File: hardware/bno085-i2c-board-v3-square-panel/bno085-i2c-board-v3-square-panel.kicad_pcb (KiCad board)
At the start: 2 copper layers, 60 x 76.5 mm, 200 parts, among them J5 Conn_01x04_Pin

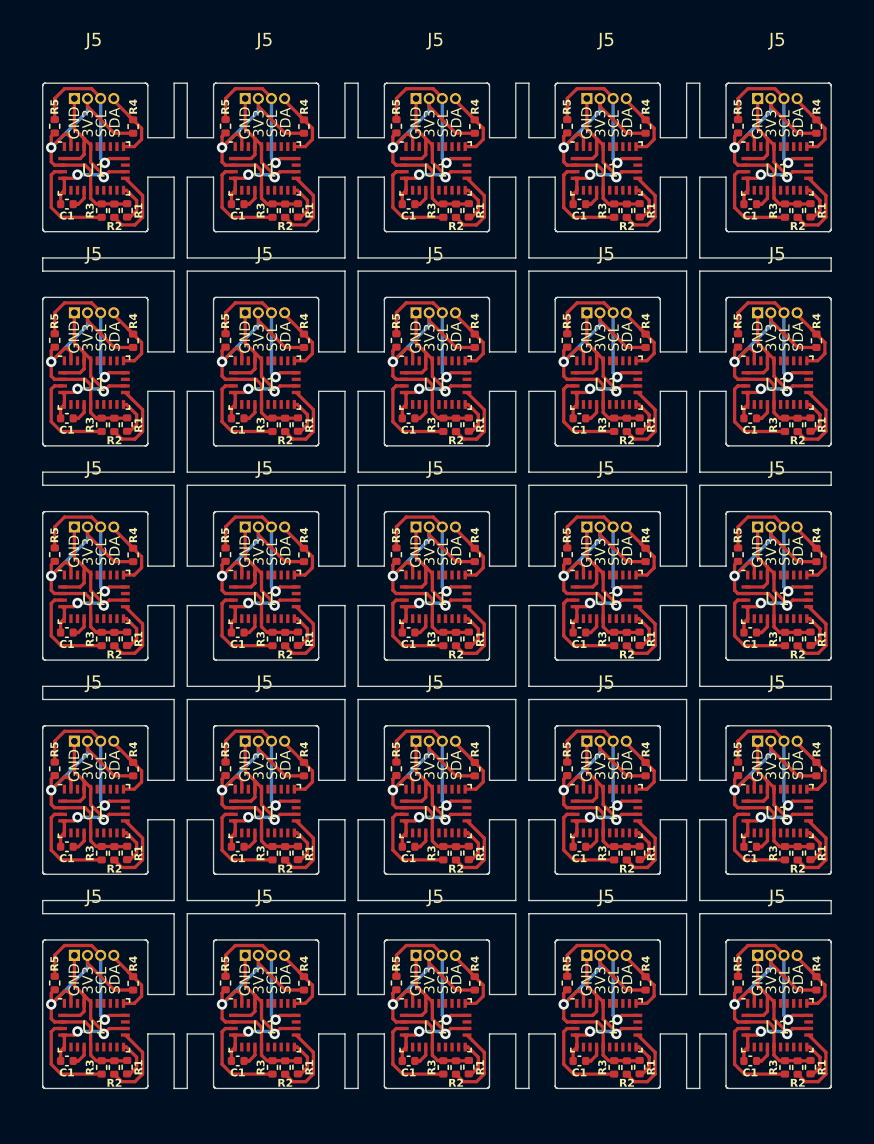
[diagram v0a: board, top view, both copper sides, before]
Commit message: square panel
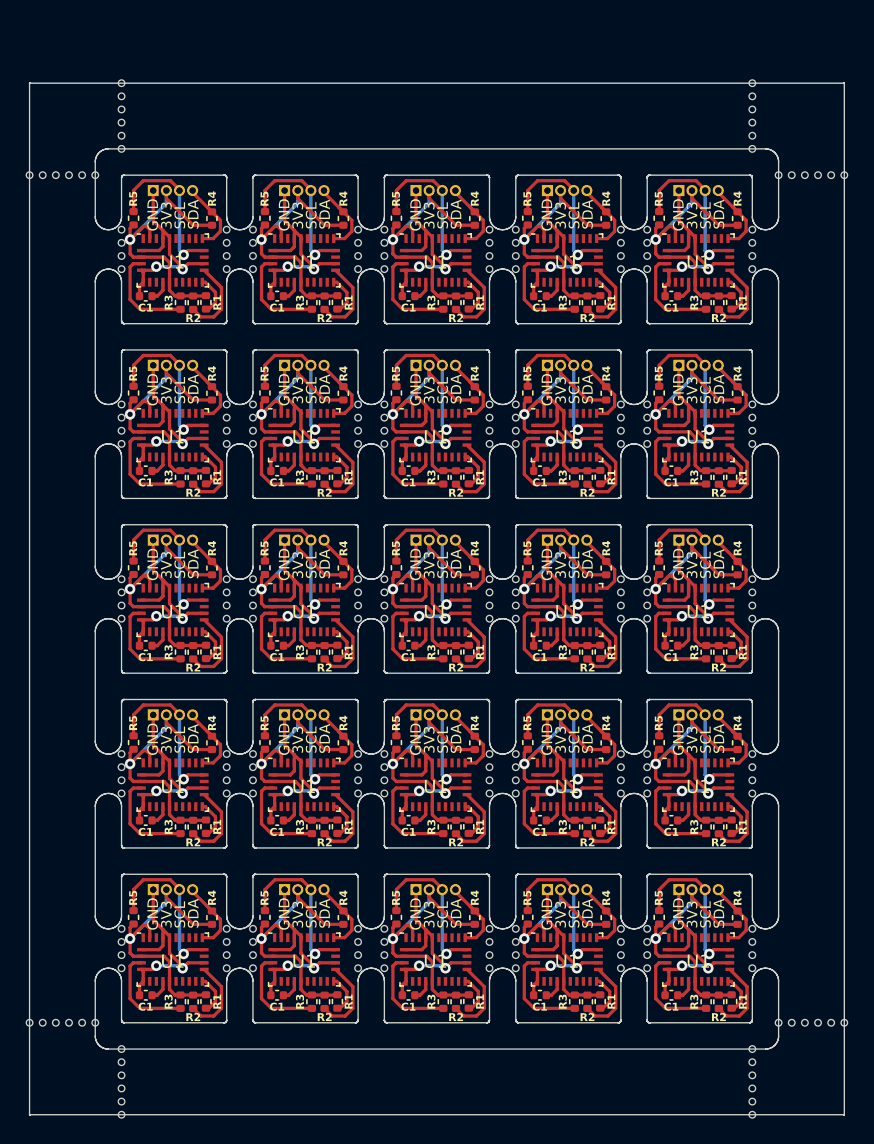
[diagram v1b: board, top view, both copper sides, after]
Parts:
- removed the C1 at (120.3, 29.2)
- removed the C1 at (172.3, 45.5)
- removed the C1 at (133.3, 94.4)
- removed the C1 at (133.3, 29.2)
- removed the C1 at (159.3, 78.1)
- removed the C1 at (159.3, 45.5)
- removed the C1 at (146.3, 94.4)
- removed the C1 at (159.3, 94.4)
- removed the C1 at (133.3, 78.1)
- removed the C1 at (133.3, 61.8)
- removed the C1 at (120.3, 61.8)
- removed the C1 at (120.3, 94.4)
- removed the C1 at (159.3, 29.2)
- removed the C1 at (172.3, 61.8)
- removed the C1 at (133.3, 45.5)
- removed the C1 at (172.3, 29.2)
- removed the C1 at (146.3, 45.5)
- removed the C1 at (120.3, 45.5)
- removed the C1 at (146.3, 61.8)
- removed the C1 at (172.3, 78.1)
- removed the C1 at (172.3, 94.4)
- removed the C1 at (146.3, 29.2)
- removed the C1 at (159.3, 61.8)
- removed the C1 at (120.3, 78.1)
- removed the C1 at (146.3, 78.1)
- removed the J5 at (172.9, 53.8)
- removed the J5 at (159.9, 37.5)
- removed the J5 at (159.9, 53.8)
- removed the J5 at (133.9, 53.8)
- removed the J5 at (120.9, 37.5)
- removed the J5 at (133.9, 37.5)
- removed the J5 at (133.9, 86.4)
- removed the J5 at (146.9, 86.4)
- removed the J5 at (172.9, 86.4)
- removed the J5 at (146.9, 53.8)
- removed the J5 at (172.9, 21.2)
- removed the J5 at (172.9, 70.1)
- removed the J5 at (146.9, 70.1)
- removed the J5 at (159.9, 70.1)
- removed the J5 at (120.9, 53.8)
- removed the J5 at (133.9, 21.2)
- removed the J5 at (120.9, 21.2)
- removed the J5 at (172.9, 37.5)
- removed the J5 at (120.9, 70.1)
- removed the J5 at (133.9, 70.1)
- removed the J5 at (146.9, 21.2)
- removed the J5 at (159.9, 86.4)
- removed the J5 at (120.9, 86.4)
- removed the J5 at (159.9, 21.2)
- removed the J5 at (146.9, 37.5)
- removed the R1 at (150.9, 78.6)
- removed the R1 at (163.9, 46.0)
- removed the R1 at (163.9, 62.3)
- removed the R1 at (124.9, 29.7)
- removed the R1 at (137.9, 78.6)
- removed the R1 at (124.9, 46.0)
- removed the R1 at (137.9, 46.0)
- removed the R1 at (176.9, 46.0)
- removed the R1 at (137.9, 62.3)
- removed the R1 at (124.9, 78.6)
- removed the R1 at (163.9, 78.6)
- removed the R1 at (150.9, 62.3)
- removed the R1 at (176.9, 29.7)
- removed the R1 at (163.9, 29.7)
- removed the R1 at (176.9, 78.6)
- removed the R1 at (150.9, 29.7)
- removed the R1 at (176.9, 94.9)
- removed the R1 at (176.9, 62.3)
- removed the R1 at (137.9, 29.7)
- removed the R1 at (150.9, 94.9)
- removed the R1 at (163.9, 94.9)
- removed the R1 at (124.9, 62.3)
- removed the R1 at (150.9, 46.0)
- removed the R1 at (124.9, 94.9)
- removed the R1 at (137.9, 94.9)
- removed the R2 at (163.0, 94.9)
- removed the R2 at (124.0, 46.0)
- removed the R2 at (124.0, 94.9)
- removed the R2 at (137.0, 46.0)
- removed the R2 at (137.0, 29.7)
- removed the R2 at (150.0, 94.9)
- removed the R2 at (176.0, 94.9)
- removed the R2 at (137.0, 62.3)
- removed the R2 at (124.0, 62.3)
- removed the R2 at (150.0, 29.7)
- removed the R2 at (176.0, 78.6)
- removed the R2 at (176.0, 46.0)
- removed the R2 at (137.0, 94.9)
- removed the R2 at (150.0, 78.6)
- removed the R2 at (124.0, 78.6)
- removed the R2 at (163.0, 46.0)
- removed the R2 at (150.0, 62.3)
- removed the R2 at (124.0, 29.7)
- removed the R2 at (163.0, 62.3)
- removed the R2 at (176.0, 62.3)
- removed the R2 at (163.0, 78.6)
- removed the R2 at (150.0, 46.0)
- removed the R2 at (137.0, 78.6)
- removed the R2 at (176.0, 29.7)
- removed the R2 at (163.0, 29.7)
- removed the R3 at (149.0, 94.9)
- removed the R3 at (149.0, 62.3)
- removed the R3 at (136.0, 29.7)
- removed the R3 at (162.0, 62.3)
- removed the R3 at (123.0, 62.3)
- removed the R3 at (149.0, 29.7)
- removed the R3 at (162.0, 29.7)
- removed the R3 at (123.0, 94.9)
- removed the R3 at (136.0, 94.9)
- removed the R3 at (175.0, 78.6)
- removed the R3 at (123.0, 46.0)
- removed the R3 at (123.0, 78.6)
- removed the R3 at (123.0, 29.7)
- removed the R3 at (175.0, 62.3)
- removed the R3 at (162.0, 78.6)
- removed the R3 at (136.0, 46.0)
- removed the R3 at (162.0, 46.0)
- removed the R3 at (175.0, 46.0)
- removed the R3 at (162.0, 94.9)
- removed the R3 at (149.0, 46.0)
- removed the R3 at (175.0, 94.9)
- removed the R3 at (136.0, 62.3)
- removed the R3 at (175.0, 29.7)
- removed the R3 at (149.0, 78.6)
- removed the R3 at (136.0, 78.6)
- removed the R4 at (164.4, 55.9)
- removed the R4 at (125.4, 55.9)
- removed the R4 at (164.4, 39.6)
- removed the R4 at (125.4, 88.5)
- removed the R4 at (125.4, 72.2)
- removed the R4 at (138.4, 39.6)
- removed the R4 at (177.4, 39.6)
- removed the R4 at (177.4, 23.3)
- removed the R4 at (151.4, 88.5)
- removed the R4 at (125.4, 23.3)
- removed the R4 at (151.4, 39.6)
- removed the R4 at (138.4, 23.3)
- removed the R4 at (151.4, 72.2)
- removed the R4 at (151.4, 55.9)
- removed the R4 at (177.4, 88.5)
- removed the R4 at (164.4, 72.2)
- removed the R4 at (177.4, 55.9)
- removed the R4 at (125.4, 39.6)
- removed the R4 at (151.4, 23.3)
- removed the R4 at (164.4, 23.3)
- removed the R4 at (138.4, 72.2)
- removed the R4 at (138.4, 88.5)
- removed the R4 at (177.4, 72.2)
- removed the R4 at (164.4, 88.5)
- removed the R4 at (138.4, 55.9)
- removed the R5 at (171.4, 55.9)
- removed the R5 at (132.4, 39.6)
- removed the R5 at (158.4, 23.3)
- removed the R5 at (158.4, 55.9)
- removed the R5 at (132.4, 55.9)
- removed the R5 at (171.4, 72.2)
- removed the R5 at (145.4, 23.3)
- removed the R5 at (119.4, 55.9)
- removed the R5 at (119.4, 39.6)
- removed the R5 at (132.4, 72.2)
- removed the R5 at (132.4, 88.5)
- removed the R5 at (171.4, 23.3)
- removed the R5 at (119.4, 88.5)
- removed the R5 at (171.4, 88.5)
- removed the R5 at (145.4, 72.2)
- removed the R5 at (119.4, 23.3)
- removed the R5 at (145.4, 39.6)
- removed the R5 at (132.4, 23.3)
- removed the R5 at (158.4, 39.6)
- removed the R5 at (145.4, 88.5)
- removed the R5 at (171.4, 39.6)
- removed the R5 at (158.4, 88.5)
- removed the R5 at (145.4, 55.9)
- removed the R5 at (158.4, 72.2)
- removed the R5 at (119.4, 72.2)
- removed the U1 at (174.4, 26.5)
- removed the U1 at (174.4, 42.8)
- removed the U1 at (135.4, 59.1)
- removed the U1 at (148.4, 91.7)
- removed the U1 at (122.4, 59.1)
- removed the U1 at (148.4, 75.4)
- removed the U1 at (161.4, 42.8)
- removed the U1 at (135.4, 26.5)
- removed the U1 at (148.4, 59.1)
- removed the U1 at (161.4, 59.1)
- removed the U1 at (122.4, 26.5)
- removed the U1 at (135.4, 75.4)
- removed the U1 at (174.4, 59.1)
- removed the U1 at (148.4, 26.5)
- removed the U1 at (122.4, 42.8)
- removed the U1 at (135.4, 42.8)
- removed the U1 at (135.4, 91.7)
- removed the U1 at (161.4, 91.7)
- removed the U1 at (161.4, 75.4)
- removed the U1 at (174.4, 91.7)
- removed the U1 at (161.4, 26.5)
- removed the U1 at (174.4, 75.4)
- removed the U1 at (122.4, 91.7)
- removed the U1 at (148.4, 42.8)
- removed the U1 at (122.4, 75.4)
- added C1: 0.1uF, Capacitor_SMD:C_0402_1005Metric, F.Cu at (156.3, 89.4)
- added C1: 0.1uF, Capacitor_SMD:C_0402_1005Metric, F.Cu at (146.3, 89.4)
- added C1: 0.1uF, Capacitor_SMD:C_0402_1005Metric, F.Cu at (126.3, 76.1)
- added C1: 0.1uF, Capacitor_SMD:C_0402_1005Metric, F.Cu at (146.3, 76.1)
- added C1: 0.1uF, Capacitor_SMD:C_0402_1005Metric, F.Cu at (146.3, 49.5)
- added C1: 0.1uF, Capacitor_SMD:C_0402_1005Metric, F.Cu at (146.3, 62.8)
- added C1: 0.1uF, Capacitor_SMD:C_0402_1005Metric, F.Cu at (126.3, 89.4)
- added C1: 0.1uF, Capacitor_SMD:C_0402_1005Metric, F.Cu at (156.3, 62.8)
- added C1: 0.1uF, Capacitor_SMD:C_0402_1005Metric, F.Cu at (136.3, 49.5)
- added C1: 0.1uF, Capacitor_SMD:C_0402_1005Metric, F.Cu at (136.3, 76.1)
- added C1: 0.1uF, Capacitor_SMD:C_0402_1005Metric, F.Cu at (136.3, 36.2)
- added C1: 0.1uF, Capacitor_SMD:C_0402_1005Metric, F.Cu at (166.3, 49.5)
- added C1: 0.1uF, Capacitor_SMD:C_0402_1005Metric, F.Cu at (166.3, 76.1)
- added C1: 0.1uF, Capacitor_SMD:C_0402_1005Metric, F.Cu at (136.3, 62.8)
- added C1: 0.1uF, Capacitor_SMD:C_0402_1005Metric, F.Cu at (136.3, 89.4)
- added C1: 0.1uF, Capacitor_SMD:C_0402_1005Metric, F.Cu at (156.3, 49.5)
- added C1: 0.1uF, Capacitor_SMD:C_0402_1005Metric, F.Cu at (146.3, 36.2)
- added C1: 0.1uF, Capacitor_SMD:C_0402_1005Metric, F.Cu at (126.3, 36.2)
- added C1: 0.1uF, Capacitor_SMD:C_0402_1005Metric, F.Cu at (166.3, 62.8)
- added C1: 0.1uF, Capacitor_SMD:C_0402_1005Metric, F.Cu at (166.3, 89.4)
- added C1: 0.1uF, Capacitor_SMD:C_0402_1005Metric, F.Cu at (126.3, 49.5)
- added C1: 0.1uF, Capacitor_SMD:C_0402_1005Metric, F.Cu at (126.3, 62.8)
- added C1: 0.1uF, Capacitor_SMD:C_0402_1005Metric, F.Cu at (166.3, 36.2)
- added C1: 0.1uF, Capacitor_SMD:C_0402_1005Metric, F.Cu at (156.3, 76.1)
- added C1: 0.1uF, Capacitor_SMD:C_0402_1005Metric, F.Cu at (156.3, 36.2)
- added J5: Conn_01x04_Pin, Connector_PinHeader_1.00mm:PinHeader_1x04_P1.00mm_Vertical, F.Cu at (146.9, 81.4)
- added J5: Conn_01x04_Pin, Connector_PinHeader_1.00mm:PinHeader_1x04_P1.00mm_Vertical, F.Cu at (166.9, 28.2)
- added J5: Conn_01x04_Pin, Connector_PinHeader_1.00mm:PinHeader_1x04_P1.00mm_Vertical, F.Cu at (126.9, 81.4)
- added J5: Conn_01x04_Pin, Connector_PinHeader_1.00mm:PinHeader_1x04_P1.00mm_Vertical, F.Cu at (156.9, 28.2)
- added J5: Conn_01x04_Pin, Connector_PinHeader_1.00mm:PinHeader_1x04_P1.00mm_Vertical, F.Cu at (126.9, 41.5)
- added J5: Conn_01x04_Pin, Connector_PinHeader_1.00mm:PinHeader_1x04_P1.00mm_Vertical, F.Cu at (166.9, 41.5)
- added J5: Conn_01x04_Pin, Connector_PinHeader_1.00mm:PinHeader_1x04_P1.00mm_Vertical, F.Cu at (146.9, 68.1)
- added J5: Conn_01x04_Pin, Connector_PinHeader_1.00mm:PinHeader_1x04_P1.00mm_Vertical, F.Cu at (136.9, 28.2)
- added J5: Conn_01x04_Pin, Connector_PinHeader_1.00mm:PinHeader_1x04_P1.00mm_Vertical, F.Cu at (136.9, 68.1)
- added J5: Conn_01x04_Pin, Connector_PinHeader_1.00mm:PinHeader_1x04_P1.00mm_Vertical, F.Cu at (146.9, 41.5)
- added J5: Conn_01x04_Pin, Connector_PinHeader_1.00mm:PinHeader_1x04_P1.00mm_Vertical, F.Cu at (166.9, 81.4)
- added J5: Conn_01x04_Pin, Connector_PinHeader_1.00mm:PinHeader_1x04_P1.00mm_Vertical, F.Cu at (146.9, 54.8)
- added J5: Conn_01x04_Pin, Connector_PinHeader_1.00mm:PinHeader_1x04_P1.00mm_Vertical, F.Cu at (156.9, 81.4)
- added J5: Conn_01x04_Pin, Connector_PinHeader_1.00mm:PinHeader_1x04_P1.00mm_Vertical, F.Cu at (146.9, 28.2)
- added J5: Conn_01x04_Pin, Connector_PinHeader_1.00mm:PinHeader_1x04_P1.00mm_Vertical, F.Cu at (156.9, 54.8)
- added J5: Conn_01x04_Pin, Connector_PinHeader_1.00mm:PinHeader_1x04_P1.00mm_Vertical, F.Cu at (126.9, 54.8)
- added J5: Conn_01x04_Pin, Connector_PinHeader_1.00mm:PinHeader_1x04_P1.00mm_Vertical, F.Cu at (136.9, 81.4)
- added J5: Conn_01x04_Pin, Connector_PinHeader_1.00mm:PinHeader_1x04_P1.00mm_Vertical, F.Cu at (156.9, 68.1)
- added J5: Conn_01x04_Pin, Connector_PinHeader_1.00mm:PinHeader_1x04_P1.00mm_Vertical, F.Cu at (126.9, 28.2)
- added J5: Conn_01x04_Pin, Connector_PinHeader_1.00mm:PinHeader_1x04_P1.00mm_Vertical, F.Cu at (136.9, 41.5)
- added J5: Conn_01x04_Pin, Connector_PinHeader_1.00mm:PinHeader_1x04_P1.00mm_Vertical, F.Cu at (126.9, 68.1)
- added J5: Conn_01x04_Pin, Connector_PinHeader_1.00mm:PinHeader_1x04_P1.00mm_Vertical, F.Cu at (166.9, 68.1)
- added J5: Conn_01x04_Pin, Connector_PinHeader_1.00mm:PinHeader_1x04_P1.00mm_Vertical, F.Cu at (166.9, 54.8)
- added J5: Conn_01x04_Pin, Connector_PinHeader_1.00mm:PinHeader_1x04_P1.00mm_Vertical, F.Cu at (156.9, 41.5)
- added J5: Conn_01x04_Pin, Connector_PinHeader_1.00mm:PinHeader_1x04_P1.00mm_Vertical, F.Cu at (136.9, 54.8)
- added R1: 2.2k, Resistor_SMD:R_0402_1005Metric, F.Cu at (170.9, 89.9)
- added R1: 2.2k, Resistor_SMD:R_0402_1005Metric, F.Cu at (170.9, 63.3)
- added R1: 2.2k, Resistor_SMD:R_0402_1005Metric, F.Cu at (140.9, 36.7)
- added R1: 2.2k, Resistor_SMD:R_0402_1005Metric, F.Cu at (160.9, 76.6)
- added R1: 2.2k, Resistor_SMD:R_0402_1005Metric, F.Cu at (150.9, 36.7)
- added R1: 2.2k, Resistor_SMD:R_0402_1005Metric, F.Cu at (140.9, 50.0)
- added R1: 2.2k, Resistor_SMD:R_0402_1005Metric, F.Cu at (150.9, 76.6)
- added R1: 2.2k, Resistor_SMD:R_0402_1005Metric, F.Cu at (140.9, 76.6)
- added R1: 2.2k, Resistor_SMD:R_0402_1005Metric, F.Cu at (130.9, 76.6)
- added R1: 2.2k, Resistor_SMD:R_0402_1005Metric, F.Cu at (130.9, 50.0)
- added R1: 2.2k, Resistor_SMD:R_0402_1005Metric, F.Cu at (170.9, 36.7)
- added R1: 2.2k, Resistor_SMD:R_0402_1005Metric, F.Cu at (140.9, 89.9)
- added R1: 2.2k, Resistor_SMD:R_0402_1005Metric, F.Cu at (130.9, 36.7)
- added R1: 2.2k, Resistor_SMD:R_0402_1005Metric, F.Cu at (160.9, 63.3)
- added R1: 2.2k, Resistor_SMD:R_0402_1005Metric, F.Cu at (160.9, 50.0)
- added R1: 2.2k, Resistor_SMD:R_0402_1005Metric, F.Cu at (170.9, 76.6)
- added R1: 2.2k, Resistor_SMD:R_0402_1005Metric, F.Cu at (140.9, 63.3)
- added R1: 2.2k, Resistor_SMD:R_0402_1005Metric, F.Cu at (160.9, 89.9)
- added R1: 2.2k, Resistor_SMD:R_0402_1005Metric, F.Cu at (150.9, 89.9)
- added R1: 2.2k, Resistor_SMD:R_0402_1005Metric, F.Cu at (170.9, 50.0)
- added R1: 2.2k, Resistor_SMD:R_0402_1005Metric, F.Cu at (150.9, 63.3)
- added R1: 2.2k, Resistor_SMD:R_0402_1005Metric, F.Cu at (160.9, 36.7)
- added R1: 2.2k, Resistor_SMD:R_0402_1005Metric, F.Cu at (150.9, 50.0)
- added R1: 2.2k, Resistor_SMD:R_0402_1005Metric, F.Cu at (130.9, 63.3)
- added R1: 2.2k, Resistor_SMD:R_0402_1005Metric, F.Cu at (130.9, 89.9)
- added R2: 2.2k, Resistor_SMD:R_0402_1005Metric, F.Cu at (160.0, 76.6)
- added R2: 2.2k, Resistor_SMD:R_0402_1005Metric, F.Cu at (160.0, 89.9)
- added R2: 2.2k, Resistor_SMD:R_0402_1005Metric, F.Cu at (150.0, 63.3)
- added R2: 2.2k, Resistor_SMD:R_0402_1005Metric, F.Cu at (170.0, 76.6)
- added R2: 2.2k, Resistor_SMD:R_0402_1005Metric, F.Cu at (140.0, 89.9)
- added R2: 2.2k, Resistor_SMD:R_0402_1005Metric, F.Cu at (150.0, 76.6)
- added R2: 2.2k, Resistor_SMD:R_0402_1005Metric, F.Cu at (140.0, 50.0)
- added R2: 2.2k, Resistor_SMD:R_0402_1005Metric, F.Cu at (160.0, 50.0)
- added R2: 2.2k, Resistor_SMD:R_0402_1005Metric, F.Cu at (170.0, 63.3)
- added R2: 2.2k, Resistor_SMD:R_0402_1005Metric, F.Cu at (130.0, 76.6)
- added R2: 2.2k, Resistor_SMD:R_0402_1005Metric, F.Cu at (150.0, 36.7)
- added R2: 2.2k, Resistor_SMD:R_0402_1005Metric, F.Cu at (130.0, 36.7)
- added R2: 2.2k, Resistor_SMD:R_0402_1005Metric, F.Cu at (140.0, 76.6)
- added R2: 2.2k, Resistor_SMD:R_0402_1005Metric, F.Cu at (170.0, 89.9)
- added R2: 2.2k, Resistor_SMD:R_0402_1005Metric, F.Cu at (160.0, 63.3)
- added R2: 2.2k, Resistor_SMD:R_0402_1005Metric, F.Cu at (140.0, 63.3)
- added R2: 2.2k, Resistor_SMD:R_0402_1005Metric, F.Cu at (130.0, 89.9)
- added R2: 2.2k, Resistor_SMD:R_0402_1005Metric, F.Cu at (170.0, 50.0)
- added R2: 2.2k, Resistor_SMD:R_0402_1005Metric, F.Cu at (160.0, 36.7)
- added R2: 2.2k, Resistor_SMD:R_0402_1005Metric, F.Cu at (150.0, 50.0)
- added R2: 2.2k, Resistor_SMD:R_0402_1005Metric, F.Cu at (130.0, 63.3)
- added R2: 2.2k, Resistor_SMD:R_0402_1005Metric, F.Cu at (170.0, 36.7)
- added R2: 2.2k, Resistor_SMD:R_0402_1005Metric, F.Cu at (140.0, 36.7)
- added R2: 2.2k, Resistor_SMD:R_0402_1005Metric, F.Cu at (150.0, 89.9)
- added R2: 2.2k, Resistor_SMD:R_0402_1005Metric, F.Cu at (130.0, 50.0)
- added R3: 10k, Resistor_SMD:R_0402_1005Metric, F.Cu at (169.0, 63.3)
- added R3: 10k, Resistor_SMD:R_0402_1005Metric, F.Cu at (129.0, 50.0)
- added R3: 10k, Resistor_SMD:R_0402_1005Metric, F.Cu at (169.0, 76.6)
- added R3: 10k, Resistor_SMD:R_0402_1005Metric, F.Cu at (139.0, 50.0)
- added R3: 10k, Resistor_SMD:R_0402_1005Metric, F.Cu at (129.0, 63.3)
- added R3: 10k, Resistor_SMD:R_0402_1005Metric, F.Cu at (139.0, 63.3)
- added R3: 10k, Resistor_SMD:R_0402_1005Metric, F.Cu at (149.0, 50.0)
- added R3: 10k, Resistor_SMD:R_0402_1005Metric, F.Cu at (169.0, 89.9)
- added R3: 10k, Resistor_SMD:R_0402_1005Metric, F.Cu at (129.0, 36.7)
- added R3: 10k, Resistor_SMD:R_0402_1005Metric, F.Cu at (159.0, 50.0)
- added R3: 10k, Resistor_SMD:R_0402_1005Metric, F.Cu at (159.0, 76.6)
- added R3: 10k, Resistor_SMD:R_0402_1005Metric, F.Cu at (159.0, 63.3)
- added R3: 10k, Resistor_SMD:R_0402_1005Metric, F.Cu at (149.0, 89.9)
- added R3: 10k, Resistor_SMD:R_0402_1005Metric, F.Cu at (159.0, 89.9)
- added R3: 10k, Resistor_SMD:R_0402_1005Metric, F.Cu at (169.0, 50.0)
- added R3: 10k, Resistor_SMD:R_0402_1005Metric, F.Cu at (169.0, 36.7)
- added R3: 10k, Resistor_SMD:R_0402_1005Metric, F.Cu at (129.0, 76.6)
- added R3: 10k, Resistor_SMD:R_0402_1005Metric, F.Cu at (139.0, 89.9)
- added R3: 10k, Resistor_SMD:R_0402_1005Metric, F.Cu at (159.0, 36.7)
- added R3: 10k, Resistor_SMD:R_0402_1005Metric, F.Cu at (139.0, 76.6)
- added R3: 10k, Resistor_SMD:R_0402_1005Metric, F.Cu at (149.0, 63.3)
- added R3: 10k, Resistor_SMD:R_0402_1005Metric, F.Cu at (149.0, 76.6)
- added R3: 10k, Resistor_SMD:R_0402_1005Metric, F.Cu at (149.0, 36.7)
- added R3: 10k, Resistor_SMD:R_0402_1005Metric, F.Cu at (139.0, 36.7)
- added R3: 10k, Resistor_SMD:R_0402_1005Metric, F.Cu at (129.0, 89.9)
- added R4: 2.2k, Resistor_SMD:R_0402_1005Metric, F.Cu at (131.4, 56.9)
- added R4: 2.2k, Resistor_SMD:R_0402_1005Metric, F.Cu at (131.4, 83.5)
- added R4: 2.2k, Resistor_SMD:R_0402_1005Metric, F.Cu at (151.4, 30.3)
- added R4: 2.2k, Resistor_SMD:R_0402_1005Metric, F.Cu at (141.4, 70.2)
- added R4: 2.2k, Resistor_SMD:R_0402_1005Metric, F.Cu at (161.4, 70.2)
- added R4: 2.2k, Resistor_SMD:R_0402_1005Metric, F.Cu at (161.4, 83.5)
- added R4: 2.2k, Resistor_SMD:R_0402_1005Metric, F.Cu at (151.4, 56.9)
- added R4: 2.2k, Resistor_SMD:R_0402_1005Metric, F.Cu at (141.4, 30.3)
- added R4: 2.2k, Resistor_SMD:R_0402_1005Metric, F.Cu at (161.4, 56.9)
- added R4: 2.2k, Resistor_SMD:R_0402_1005Metric, F.Cu at (171.4, 70.2)
- added R4: 2.2k, Resistor_SMD:R_0402_1005Metric, F.Cu at (131.4, 70.2)
- added R4: 2.2k, Resistor_SMD:R_0402_1005Metric, F.Cu at (161.4, 30.3)
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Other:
- board size 60 x 76.5 mm -> 62 x 78.5 mm

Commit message: panels and board metadata
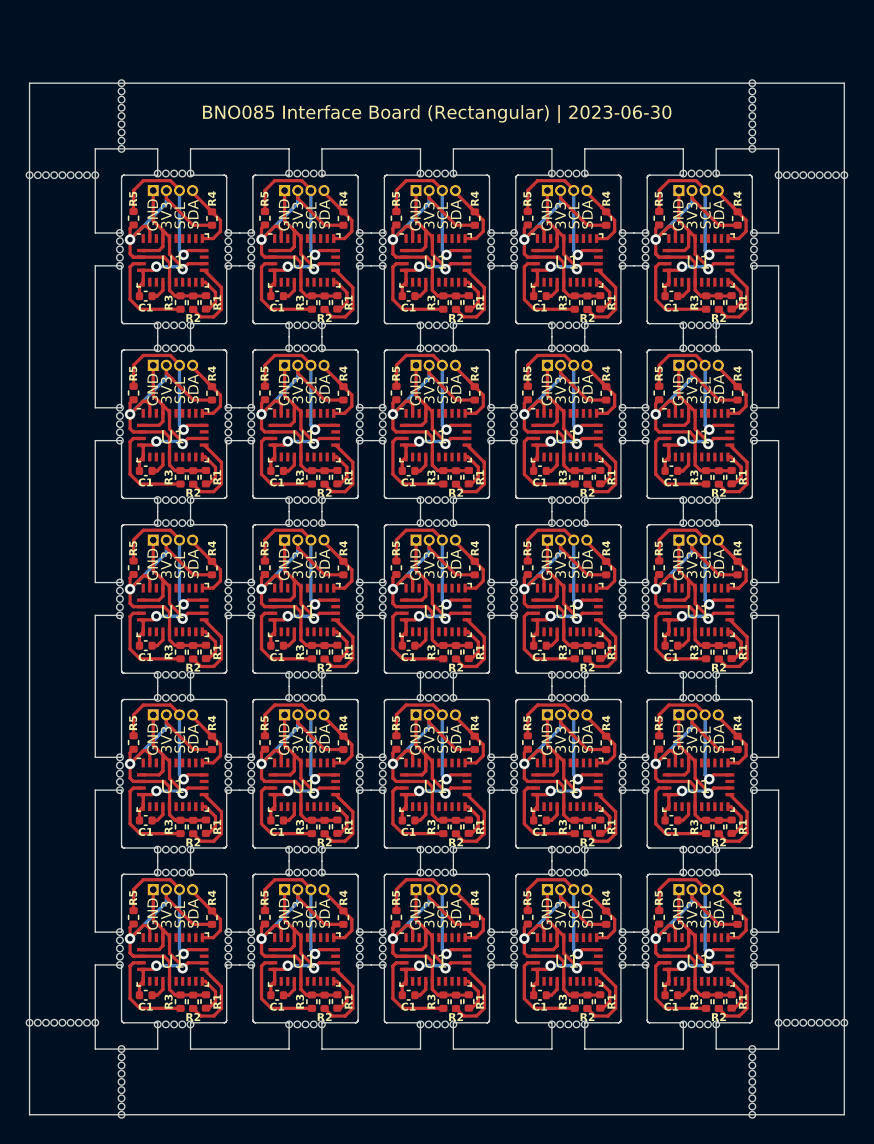
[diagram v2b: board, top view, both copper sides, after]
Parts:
- removed the REF** at (152.5, 32.1)
- removed the REF** at (134.5, 60.8)
- removed the REF** at (175.5, 27.0)
- removed the REF** at (142.5, 33.1)
- removed the REF** at (162.5, 58.8)
- removed the REF** at (164.5, 85.3)
- removed the REF** at (142.5, 47.5)
- removed the REF** at (134.5, 47.5)
- removed the REF** at (142.5, 72.0)
- removed the REF** at (124.5, 21.0)
- removed the REF** at (154.5, 74.0)
- removed the REF** at (164.5, 72.0)
- removed the REF** at (132.5, 71.0)
- removed the REF** at (144.5, 72.0)
- removed the REF** at (134.5, 86.3)
- removed the REF** at (119.5, 91.5)
- removed the REF** at (124.5, 34.1)
- removed the REF** at (144.5, 85.3)
- removed the REF** at (142.5, 31.1)
- removed the REF** at (134.5, 74.0)
- removed the REF** at (152.5, 47.5)
- removed the REF** at (152.5, 73.0)
- removed the REF** at (164.5, 87.3)
- removed the REF** at (162.5, 74.0)
- removed the REF** at (172.5, 94.5)
- removed the REF** at (132.5, 57.8)
- removed the REF** at (124.5, 86.3)
- removed the REF** at (132.5, 47.5)
- removed the REF** at (152.5, 59.8)
- removed the REF** at (172.5, 34.1)
- removed the REF** at (164.5, 46.5)
- removed the REF** at (144.5, 59.8)
- removed the REF** at (124.5, 59.8)
- removed the REF** at (162.5, 59.8)
- removed the REF** at (162.5, 33.1)
- removed the REF** at (164.5, 57.8)
- removed the REF** at (162.5, 45.5)
- removed the REF** at (152.5, 58.8)
- removed the REF** at (121.5, 91.5)
- removed the REF** at (124.5, 96.5)
- removed the REF** at (162.5, 60.8)
- removed the REF** at (172.5, 44.5)
- removed the REF** at (124.5, 45.5)
- removed the REF** at (124.5, 94.5)
- removed the REF** at (172.5, 71.0)
- removed the REF** at (154.5, 44.5)
- removed the REF** at (144.5, 86.3)
- removed the REF** at (144.5, 47.5)
- removed the REF** at (152.5, 71.0)
- removed the REF** at (142.5, 60.8)
- removed the REF** at (154.5, 87.3)
- removed the REF** at (172.5, 33.1)
- removed the REF** at (124.5, 57.8)
- removed the REF** at (134.5, 57.8)
- removed the REF** at (162.5, 34.1)
- removed the REF** at (124.5, 46.5)
- removed the REF** at (142.5, 87.3)
- removed the REF** at (162.5, 72.0)
- removed the REF** at (152.5, 87.3)
- removed the REF** at (172.5, 84.3)
- removed the REF** at (177.5, 27.0)
- removed the REF** at (134.5, 32.1)
- removed the REF** at (164.5, 32.1)
- removed the REF** at (134.5, 71.0)
- removed the REF** at (134.5, 44.5)
- removed the REF** at (164.5, 58.8)
- removed the REF** at (132.5, 31.1)
- removed the REF** at (172.5, 59.8)
- removed the REF** at (172.5, 57.8)
- removed the REF** at (144.5, 84.3)
- removed the REF** at (152.5, 60.8)
- removed the REF** at (124.5, 31.1)
- removed the REF** at (162.5, 47.5)
- removed the REF** at (124.5, 24.0)
- removed the REF** at (152.5, 57.8)
- removed the REF** at (132.5, 34.1)
- removed the REF** at (154.5, 72.0)
- removed the REF** at (162.5, 44.5)
- removed the REF** at (132.5, 33.1)
- removed the REF** at (154.5, 85.3)
- removed the REF** at (124.5, 60.8)
- removed the REF** at (132.5, 85.3)
- removed the REF** at (132.5, 45.5)
- removed the REF** at (172.5, 23.0)
- removed the REF** at (172.5, 95.5)
- removed the REF** at (164.5, 86.3)
- removed the REF** at (124.5, 95.5)
- removed the REF** at (124.5, 97.5)
- removed the REF** at (172.5, 45.5)
- removed the REF** at (134.5, 45.5)
- removed the REF** at (154.5, 32.1)
- removed the REF** at (132.5, 86.3)
- removed the REF** at (152.5, 74.0)
- removed the REF** at (152.5, 72.0)
- removed the REF** at (142.5, 34.1)
- removed the REF** at (164.5, 73.0)
- removed the REF** at (178.5, 27.0)
- removed the REF** at (172.5, 31.1)
- removed the REF** at (162.5, 84.3)
- removed the REF** at (118.5, 91.5)
- removed the REF** at (152.5, 44.5)
- removed the REF** at (144.5, 87.3)
- removed the REF** at (121.5, 27.0)
- removed the REF** at (132.5, 74.0)
- removed the REF** at (142.5, 32.1)
- removed the REF** at (124.5, 74.0)
- removed the REF** at (152.5, 31.1)
- removed the REF** at (164.5, 34.1)
- removed the REF** at (134.5, 84.3)
- removed the REF** at (132.5, 58.8)
- removed the REF** at (134.5, 85.3)
- removed the REF** at (144.5, 57.8)
- removed the REF** at (144.5, 60.8)
- removed the REF** at (178.5, 91.5)
- removed the REF** at (134.5, 34.1)
- removed the REF** at (124.5, 32.1)
- removed the REF** at (144.5, 33.1)
- removed the REF** at (164.5, 74.0)
- removed the REF** at (132.5, 46.5)
- removed the REF** at (124.5, 22.0)
- removed the REF** at (154.5, 57.8)
- removed the REF** at (152.5, 34.1)
- removed the REF** at (119.5, 27.0)
- removed the REF** at (124.5, 47.5)
- removed the REF** at (142.5, 46.5)
- removed the REF** at (152.5, 84.3)
- removed the REF** at (132.5, 84.3)
- removed the REF** at (144.5, 34.1)
- removed the REF** at (164.5, 71.0)
- removed the REF** at (142.5, 74.0)
- removed the REF** at (120.5, 91.5)
- removed the REF** at (162.5, 32.1)
- removed the REF** at (154.5, 45.5)
- removed the REF** at (162.5, 46.5)
- removed the REF** at (142.5, 85.3)
- removed the REF** at (132.5, 60.8)
- removed the REF** at (162.5, 57.8)
- removed the REF** at (124.5, 23.0)
- removed the REF** at (172.5, 74.0)
- removed the REF** at (172.5, 24.0)
- removed the REF** at (142.5, 71.0)
- removed the REF** at (142.5, 59.8)
- removed the REF** at (164.5, 31.1)
- removed the REF** at (154.5, 31.1)
- removed the REF** at (144.5, 58.8)
- removed the REF** at (162.5, 71.0)
- removed the REF** at (124.5, 58.8)
- removed the REF** at (132.5, 32.1)
- removed the REF** at (164.5, 59.8)
- removed the REF** at (142.5, 86.3)
- removed the REF** at (154.5, 46.5)
- removed the REF** at (176.5, 27.0)
- removed the REF** at (154.5, 59.8)
- removed the REF** at (124.5, 71.0)
- removed the REF** at (152.5, 46.5)
- removed the REF** at (144.5, 45.5)
- removed the REF** at (162.5, 73.0)
- removed the REF** at (134.5, 33.1)
- removed the REF** at (134.5, 72.0)
- removed the REF** at (124.5, 84.3)
- removed the REF** at (172.5, 97.5)
- removed the REF** at (172.5, 47.5)
- removed the REF** at (142.5, 57.8)
- removed the REF** at (142.5, 73.0)
- removed the REF** at (162.5, 87.3)
- removed the REF** at (152.5, 33.1)
- removed the REF** at (134.5, 58.8)
- removed the REF** at (152.5, 85.3)
- removed the REF** at (134.5, 59.8)
- removed the REF** at (154.5, 47.5)
- removed the REF** at (142.5, 84.3)
- removed the REF** at (172.5, 72.0)
- removed the REF** at (144.5, 46.5)
- removed the REF** at (132.5, 44.5)
- removed the REF** at (124.5, 33.1)
- removed the REF** at (176.5, 91.5)
- removed the REF** at (164.5, 33.1)
- removed the REF** at (164.5, 84.3)
- removed the REF** at (124.5, 44.5)
- removed the REF** at (172.5, 87.3)
- removed the REF** at (132.5, 72.0)
- removed the REF** at (134.5, 31.1)
- removed the REF** at (162.5, 85.3)
- removed the REF** at (164.5, 60.8)
- removed the REF** at (132.5, 59.8)
- removed the REF** at (172.5, 46.5)
- removed the REF** at (144.5, 71.0)
- removed the REF** at (172.5, 22.0)
- removed the REF** at (154.5, 60.8)
- removed the REF** at (134.5, 87.3)
- removed the REF** at (172.5, 96.5)
- removed the REF** at (164.5, 44.5)
- removed the REF** at (162.5, 86.3)
- removed the REF** at (124.5, 87.3)
- removed the REF** at (118.5, 27.0)
- removed the REF** at (152.5, 45.5)
- removed the REF** at (177.5, 91.5)
- removed the REF** at (142.5, 45.5)
- removed the REF** at (172.5, 32.1)
- removed the REF** at (172.5, 60.8)
- removed the REF** at (142.5, 44.5)
- removed the REF** at (152.5, 86.3)
- removed the REF** at (120.5, 27.0)
- removed the REF** at (124.5, 85.3)
- removed the REF** at (132.5, 73.0)
- removed the REF** at (134.5, 73.0)
- removed the REF** at (154.5, 73.0)
- removed the REF** at (124.5, 73.0)
- removed the REF** at (154.5, 71.0)
- removed the REF** at (164.5, 47.5)
- removed the REF** at (154.5, 84.3)
- removed the REF** at (132.5, 87.3)
- removed the REF** at (172.5, 21.0)
- removed the REF** at (142.5, 58.8)
- removed the REF** at (144.5, 74.0)
- removed the REF** at (144.5, 31.1)
- removed the REF** at (144.5, 32.1)
- removed the REF** at (154.5, 58.8)
- removed the REF** at (172.5, 73.0)
- removed the REF** at (144.5, 73.0)
- removed the REF** at (134.5, 46.5)
- removed the REF** at (154.5, 33.1)
- removed the REF** at (172.5, 86.3)
- removed the REF** at (162.5, 31.1)
- removed the REF** at (175.5, 91.5)
- removed the REF** at (154.5, 34.1)
- removed the REF** at (144.5, 44.5)
- removed the REF** at (124.5, 72.0)
- removed the REF** at (154.5, 86.3)
- removed the REF** at (164.5, 45.5)
- removed the REF** at (172.5, 58.8)
- removed the REF** at (172.5, 85.3)
- added REF**: NPTH, NPTH, F.Cu at (159.1, 91.6)
- added REF**: NPTH, NPTH, F.Cu at (154.4, 58.6)
- added REF**: NPTH, NPTH, F.Cu at (152.6, 58.6)
- added REF**: NPTH, NPTH, F.Cu at (124.4, 72.5)
- added REF**: NPTH, NPTH, F.Cu at (172.5, 95.4)
- added REF**: NPTH, NPTH, F.Cu at (124.5, 97.2)
- added REF**: NPTH, NPTH, F.Cu at (144.4, 85.8)
- added REF**: NPTH, NPTH, F.Cu at (176.4, 27.0)
- added REF**: NPTH, NPTH, F.Cu at (124.5, 94.1)
- added REF**: NPTH, NPTH, F.Cu at (144.4, 87.1)
- added REF**: NPTH, NPTH, F.Cu at (167.2, 65.0)
- added REF**: NPTH, NPTH, F.Cu at (167.9, 40.2)
- added REF**: NPTH, NPTH, F.Cu at (144.4, 59.9)
- added REF**: NPTH, NPTH, F.Cu at (172.6, 85.8)
- added REF**: NPTH, NPTH, F.Cu at (158.5, 40.2)
- added REF**: NPTH, NPTH, F.Cu at (137.9, 80.1)
- added REF**: NPTH, NPTH, F.Cu at (129.1, 66.8)
- added REF**: NPTH, NPTH, F.Cu at (154.4, 71.3)
- added REF**: NPTH, NPTH, F.Cu at (169.1, 38.4)
- added REF**: NPTH, NPTH, F.Cu at (178.2, 91.5)
- added REF**: NPTH, NPTH, F.Cu at (167.2, 66.8)
- added REF**: NPTH, NPTH, F.Cu at (164.4, 45.3)
- added REF**: NPTH, NPTH, F.Cu at (152.6, 46.6)
- added REF**: NPTH, NPTH, F.Cu at (154.4, 58.0)
- added REF**: NPTH, NPTH, F.Cu at (134.4, 71.9)
- added REF**: NPTH, NPTH, F.Cu at (132.6, 58.6)
- added REF**: NPTH, NPTH, F.Cu at (149.8, 53.5)
- added REF**: NPTH, NPTH, F.Cu at (152.6, 60.5)
- added REF**: NPTH, NPTH, F.Cu at (144.4, 58.0)
- added REF**: NPTH, NPTH, F.Cu at (178.2, 27.0)
- added REF**: NPTH, NPTH, F.Cu at (157.2, 78.3)
- added REF**: NPTH, NPTH, F.Cu at (172.5, 96.6)
- added REF**: NPTH, NPTH, F.Cu at (152.6, 47.2)
- added REF**: NPTH, NPTH, F.Cu at (124.5, 24.4)
- added REF**: NPTH, NPTH, F.Cu at (127.2, 78.3)
- added REF**: NPTH, NPTH, F.Cu at (158.5, 91.6)
- added REF**: NPTH, NPTH, F.Cu at (124.5, 22.5)
- added REF**: NPTH, NPTH, F.Cu at (127.2, 65.0)
- added REF**: NPTH, NPTH, F.Cu at (144.4, 44.7)
- added REF**: NPTH, NPTH, F.Cu at (152.6, 73.8)
- added REF**: NPTH, NPTH, F.Cu at (152.6, 71.3)
- added REF**: NPTH, NPTH, F.Cu at (149.8, 51.7)
- added REF**: NPTH, NPTH, F.Cu at (159.8, 51.7)
- added REF**: NPTH, NPTH, F.Cu at (129.8, 80.1)
- added REF**: NPTH, NPTH, F.Cu at (162.6, 72.5)
- added REF**: NPTH, NPTH, F.Cu at (159.8, 78.3)
- added REF**: NPTH, NPTH, F.Cu at (157.2, 80.1)
- added REF**: NPTH, NPTH, F.Cu at (147.2, 78.3)
- added REF**: NPTH, NPTH, F.Cu at (154.4, 46.6)
- added REF**: NPTH, NPTH, F.Cu at (137.9, 40.2)
- added REF**: NPTH, NPTH, F.Cu at (142.6, 47.2)
- added REF**: NPTH, NPTH, F.Cu at (172.5, 23.1)
- added REF**: NPTH, NPTH, F.Cu at (118.1, 27.0)
- added REF**: NPTH, NPTH, F.Cu at (157.9, 66.8)
- added REF**: NPTH, NPTH, F.Cu at (132.6, 32.0)
- added REF**: NPTH, NPTH, F.Cu at (144.4, 85.2)
- added REF**: NPTH, NPTH, F.Cu at (157.9, 65.0)
- added REF**: NPTH, NPTH, F.Cu at (164.4, 71.9)
- added REF**: NPTH, NPTH, F.Cu at (158.5, 66.8)
- added REF**: NPTH, NPTH, F.Cu at (152.6, 85.8)
- added REF**: NPTH, NPTH, F.Cu at (139.1, 53.5)
- added REF**: NPTH, NPTH, F.Cu at (118.1, 91.5)
- added REF**: NPTH, NPTH, F.Cu at (128.5, 38.4)
- added REF**: NPTH, NPTH, F.Cu at (158.5, 51.7)
- added REF**: NPTH, NPTH, F.Cu at (128.5, 80.1)
- added REF**: NPTH, NPTH, F.Cu at (167.9, 66.8)
- added REF**: NPTH, NPTH, F.Cu at (134.4, 71.3)
- added REF**: NPTH, NPTH, F.Cu at (149.1, 53.5)
- added REF**: NPTH, NPTH, F.Cu at (167.2, 38.4)
- added REF**: NPTH, NPTH, F.Cu at (132.6, 87.1)
- added REF**: NPTH, NPTH, F.Cu at (142.6, 87.1)
- added REF**: NPTH, NPTH, F.Cu at (128.5, 78.3)
- added REF**: NPTH, NPTH, F.Cu at (172.6, 73.8)
- added REF**: NPTH, NPTH, F.Cu at (148.5, 53.5)
- added REF**: NPTH, NPTH, F.Cu at (137.2, 38.4)
- added REF**: NPTH, NPTH, F.Cu at (144.4, 33.9)
- added REF**: NPTH, NPTH, F.Cu at (167.2, 51.7)
- added REF**: NPTH, NPTH, F.Cu at (177.0, 91.5)
- added REF**: NPTH, NPTH, F.Cu at (177.0, 27.0)
- added REF**: NPTH, NPTH, F.Cu at (120.0, 27.0)
- added REF**: NPTH, NPTH, F.Cu at (162.6, 46.0)
- added REF**: NPTH, NPTH, F.Cu at (134.4, 86.5)
- added REF**: NPTH, NPTH, F.Cu at (148.5, 38.4)
- added REF**: NPTH, NPTH, F.Cu at (142.6, 58.6)
- added REF**: NPTH, NPTH, F.Cu at (144.4, 71.3)
- added REF**: NPTH, NPTH, F.Cu at (149.1, 26.9)
- added REF**: NPTH, NPTH, F.Cu at (164.4, 60.5)
- added REF**: NPTH, NPTH, F.Cu at (152.6, 73.2)
- added REF**: NPTH, NPTH, F.Cu at (142.6, 59.9)
- added REF**: NPTH, NPTH, F.Cu at (172.6, 44.7)
- added REF**: NPTH, NPTH, F.Cu at (127.9, 80.1)
- added REF**: NPTH, NPTH, F.Cu at (162.6, 33.3)
- added REF**: NPTH, NPTH, F.Cu at (159.1, 78.3)
- added REF**: NPTH, NPTH, F.Cu at (132.6, 31.4)
- added REF**: NPTH, NPTH, F.Cu at (169.8, 91.6)
- added REF**: NPTH, NPTH, F.Cu at (127.9, 78.3)
- added REF**: NPTH, NPTH, F.Cu at (124.4, 71.9)
- added REF**: NPTH, NPTH, F.Cu at (139.1, 65.0)
- added REF**: NPTH, NPTH, F.Cu at (154.4, 32.6)
- added REF**: NPTH, NPTH, F.Cu at (129.1, 78.3)
- added REF**: NPTH, NPTH, F.Cu at (144.4, 73.2)
- added REF**: NPTH, NPTH, F.Cu at (134.4, 44.7)
- added REF**: NPTH, NPTH, F.Cu at (164.4, 71.3)
- added REF**: NPTH, NPTH, F.Cu at (162.6, 71.3)
- added REF**: NPTH, NPTH, F.Cu at (147.9, 66.8)
- added REF**: NPTH, NPTH, F.Cu at (152.6, 87.1)
- added REF**: NPTH, NPTH, F.Cu at (132.6, 85.8)
- added REF**: NPTH, NPTH, F.Cu at (137.2, 51.7)
- added REF**: NPTH, NPTH, F.Cu at (128.5, 91.6)
- added REF**: NPTH, NPTH, F.Cu at (164.4, 85.8)
- added REF**: NPTH, NPTH, F.Cu at (134.4, 33.9)
- added REF**: NPTH, NPTH, F.Cu at (142.6, 86.5)
- added REF**: NPTH, NPTH, F.Cu at (157.9, 26.9)
- added REF**: NPTH, NPTH, F.Cu at (167.9, 91.6)
- added REF**: NPTH, NPTH, F.Cu at (132.6, 73.2)
- added REF**: NPTH, NPTH, F.Cu at (172.5, 97.2)
- added REF**: NPTH, NPTH, F.Cu at (147.2, 53.5)
- added REF**: NPTH, NPTH, F.Cu at (152.6, 31.4)
- added REF**: NPTH, NPTH, F.Cu at (142.6, 60.5)
- added REF**: NPTH, NPTH, F.Cu at (147.9, 40.2)
- added REF**: NPTH, NPTH, F.Cu at (144.4, 31.4)
- added REF**: NPTH, NPTH, F.Cu at (124.4, 46.6)
- added REF**: NPTH, NPTH, F.Cu at (138.5, 65.0)
- added REF**: NPTH, NPTH, F.Cu at (129.1, 38.4)
- added REF**: NPTH, NPTH, F.Cu at (164.4, 44.7)
- added REF**: NPTH, NPTH, F.Cu at (169.8, 80.1)
- added REF**: NPTH, NPTH, F.Cu at (159.1, 38.4)
- added REF**: NPTH, NPTH, F.Cu at (152.6, 85.2)
- added REF**: NPTH, NPTH, F.Cu at (144.4, 60.5)
- added REF**: NPTH, NPTH, F.Cu at (144.4, 46.6)
- added REF**: NPTH, NPTH, F.Cu at (127.9, 26.9)
- added REF**: NPTH, NPTH, F.Cu at (139.1, 40.2)
- added REF**: NPTH, NPTH, F.Cu at (134.4, 45.3)
- added REF**: NPTH, NPTH, F.Cu at (142.6, 73.8)
- added REF**: NPTH, NPTH, F.Cu at (162.6, 44.7)
- added REF**: NPTH, NPTH, F.Cu at (154.4, 72.5)
- added REF**: NPTH, NPTH, F.Cu at (119.4, 91.5)
- added REF**: NPTH, NPTH, F.Cu at (172.6, 73.2)
- added REF**: NPTH, NPTH, F.Cu at (127.9, 66.8)
- added REF**: NPTH, NPTH, F.Cu at (148.5, 80.1)
- added REF**: NPTH, NPTH, F.Cu at (157.9, 40.2)
- added REF**: NPTH, NPTH, F.Cu at (162.6, 84.6)
- added REF**: NPTH, NPTH, F.Cu at (169.8, 78.3)
- added REF**: NPTH, NPTH, F.Cu at (167.9, 38.4)
- added REF**: NPTH, NPTH, F.Cu at (144.4, 59.2)
- added REF**: NPTH, NPTH, F.Cu at (152.6, 32.0)
- added REF**: NPTH, NPTH, F.Cu at (167.9, 65.0)
- added REF**: NPTH, NPTH, F.Cu at (142.6, 32.6)
- added REF**: NPTH, NPTH, F.Cu at (142.6, 32.0)
- added REF**: NPTH, NPTH, F.Cu at (137.2, 26.9)
- added REF**: NPTH, NPTH, F.Cu at (154.4, 85.8)
- added REF**: NPTH, NPTH, F.Cu at (124.4, 31.4)
- added REF**: NPTH, NPTH, F.Cu at (137.2, 40.2)
- added REF**: NPTH, NPTH, F.Cu at (132.6, 33.3)
- added REF**: NPTH, NPTH, F.Cu at (127.9, 40.2)
- added REF**: NPTH, NPTH, F.Cu at (139.8, 53.5)
- added REF**: NPTH, NPTH, F.Cu at (124.4, 33.3)
- added REF**: NPTH, NPTH, F.Cu at (149.8, 65.0)
- added REF**: NPTH, NPTH, F.Cu at (124.4, 46.0)
- added REF**: NPTH, NPTH, F.Cu at (172.6, 84.6)
- added REF**: NPTH, NPTH, F.Cu at (167.2, 26.9)
- added REF**: NPTH, NPTH, F.Cu at (142.6, 58.0)
- added REF**: NPTH, NPTH, F.Cu at (164.4, 72.5)
- added REF**: NPTH, NPTH, F.Cu at (149.1, 40.2)
- added REF**: NPTH, NPTH, F.Cu at (172.6, 85.2)
- added REF**: NPTH, NPTH, F.Cu at (159.8, 53.5)
- added REF**: NPTH, NPTH, F.Cu at (129.8, 26.9)
- added REF**: NPTH, NPTH, F.Cu at (177.6, 27.0)
- added REF**: NPTH, NPTH, F.Cu at (127.2, 26.9)
- added REF**: NPTH, NPTH, F.Cu at (164.4, 59.9)
- added REF**: NPTH, NPTH, F.Cu at (121.2, 27.0)
- added REF**: NPTH, NPTH, F.Cu at (132.6, 85.2)
- added REF**: NPTH, NPTH, F.Cu at (172.6, 71.9)
- added REF**: NPTH, NPTH, F.Cu at (177.6, 91.5)
- added REF**: NPTH, NPTH, F.Cu at (142.6, 46.6)
- added REF**: NPTH, NPTH, F.Cu at (154.4, 59.2)
- added REF**: NPTH, NPTH, F.Cu at (134.4, 84.6)
- added REF**: NPTH, NPTH, F.Cu at (124.5, 95.4)
- added REF**: NPTH, NPTH, F.Cu at (144.4, 73.8)
- added REF**: NPTH, NPTH, F.Cu at (132.6, 46.6)
- added REF**: NPTH, NPTH, F.Cu at (169.1, 53.5)
- added REF**: NPTH, NPTH, F.Cu at (168.5, 26.9)
- added REF**: NPTH, NPTH, F.Cu at (132.6, 86.5)
- added REF**: NPTH, NPTH, F.Cu at (138.5, 91.6)
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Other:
- outline, holes or cut-outs redrawn
- board text added: "BNO085 Interface Board (Rectangular) | 2023-06-30"
